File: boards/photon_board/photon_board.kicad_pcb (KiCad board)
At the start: 2 copper layers, 9 parts, among them J1 TERASIC, J2 PHOTON, J3 DATA, U1 SN65LVDT34D, U2 SN65LVDT34D

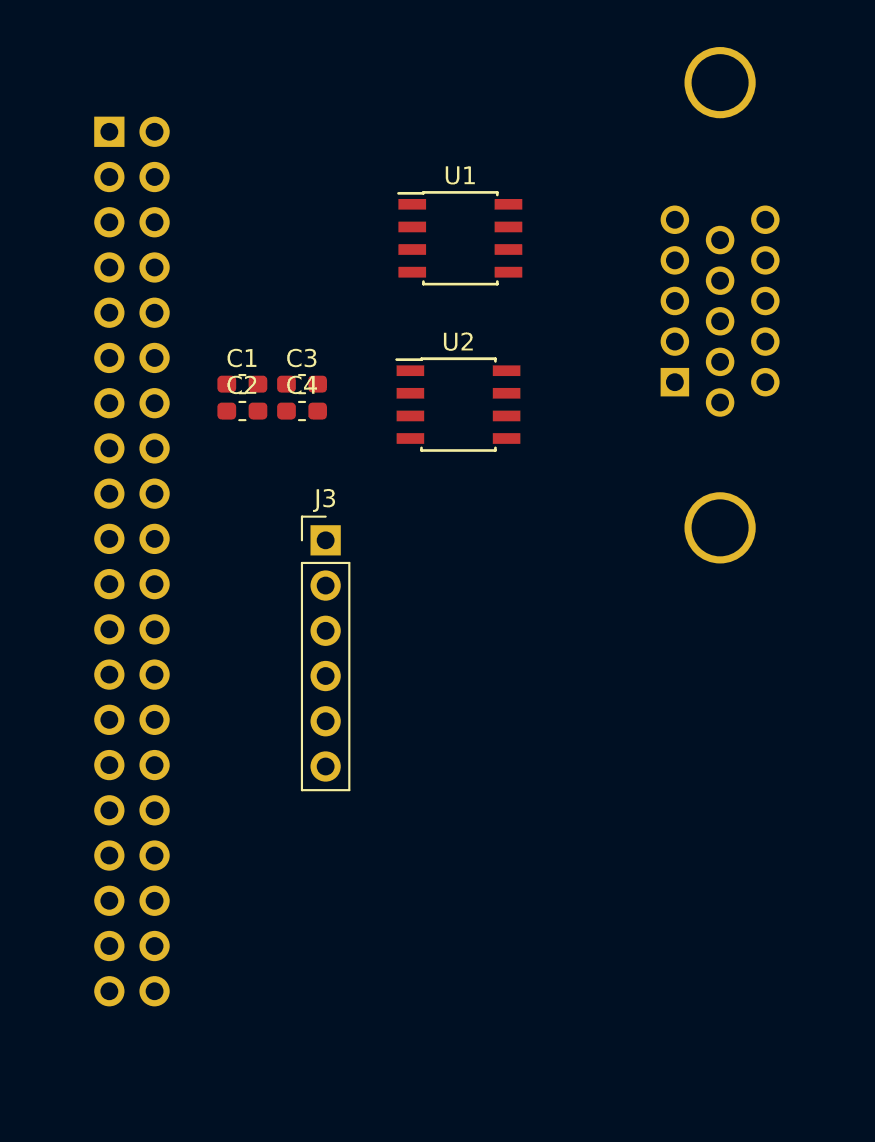
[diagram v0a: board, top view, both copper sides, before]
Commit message: route board
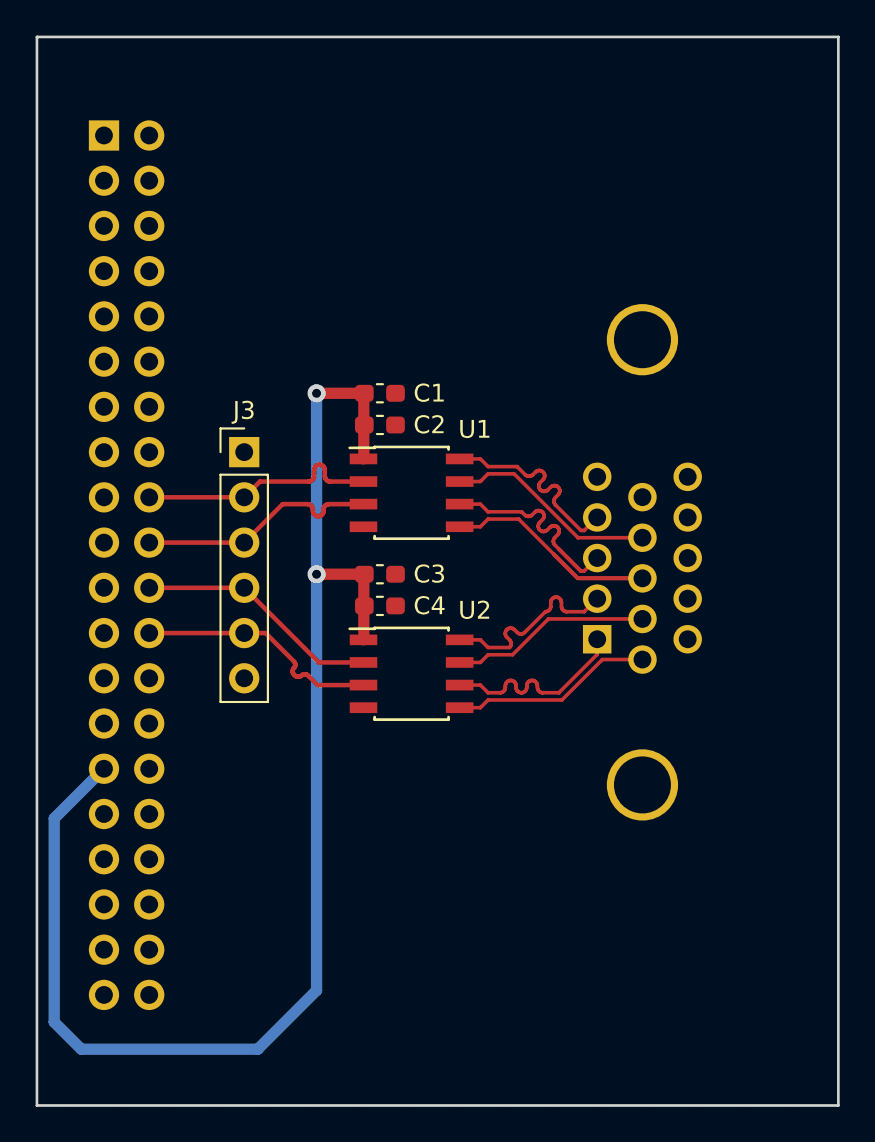
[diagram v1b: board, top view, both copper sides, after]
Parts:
- moved U2 15.3 mm to (161.0, 95.8)
- moved J2 15.1 mm to (171.5, 93.8)
- moved U1 14.6 mm to (161.0, 85.6)
- moved C4 11.8 mm to (159.3, 91.9), turned to 180 degrees
- moved C3 11.5 mm to (159.3, 90.2)
- moved C2 7.76 mm to (159.3, 81.8), turned to 180 degrees
- moved C1 7.74 mm to (159.3, 80.0)
- moved J3 6.74 mm to (151.6, 83.3)
- moved J1 0.37 mm to (143.8, 65.5)
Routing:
- net +3V3: track 0.00 -> 78.4 mm, vias 0 -> 2
- net /DATA2_OUT-: track 0.00 -> 17.4 mm
- net /DATA_SYNC: track 0.00 -> 13.8 mm
- net /DATA1_OUT: track 0.00 -> 13.8 mm
- net /DATA_CLK: track 0.00 -> 13.8 mm
- net /DATA2_OUT: track 0.00 -> 13.8 mm
- net /DATA2_OUT+: track 0.00 -> 13.6 mm
- net /DATA_CLK+: track 0.00 -> 11.9 mm
- net /DATA_CLK-: track 0.00 -> 11.9 mm
- net /DATA_SYNC+: track 0.00 -> 11.4 mm
- net /DATA_SYNC-: track 0.00 -> 11.4 mm
- net /DATA1_OUT+: track 0.00 -> 11.3 mm
- net /DATA1_OUT-: track 0.00 -> 11.3 mm
- added copper zone on B.Cu, net GND
- added copper zone on F.Cu, net GND
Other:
- board outline added: 45 x 60 mm
- net class Default: via_dia 0.8 -> 0.508; via_drill 0.4 -> 0.254
- rule via_min_drill: 0.3 -> 0.254
- rule via_min_size: 0 -> 0.508
